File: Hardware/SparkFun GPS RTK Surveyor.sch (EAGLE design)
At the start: 122 parts, among them J13 Internal, J16 microSD, J17 Qwiic Right Angle, J3 USB Female Type C Connector, J4 External, J5 USB Female Type C Connector, Q1 DMC2700UDM, Q10 20V/0.2A/8MHz/1.2Ω/1Vth, Q2 MBT3904DW1T1, Q3 20V/0.2A/8MHz/1.2Ω/1Vth, Q4 20V/0.2A/8MHz/1.2Ω/1Vth, Q7 20V/0.2A/8MHz/1.2Ω/1Vth, Q9 20V/0.2A/8MHz/1.2Ω/1Vth, U1 74HC4052D, U10 MCP73833, U13 9DoF IMU, U14 1.8V/100mA, U2 AP2112K-3.3, U3 U-BLOX_ZED-F9P, U4 ADP160, U5 ESP-WROOM-32NARROW, U6 CH340C, U7 MAX17048

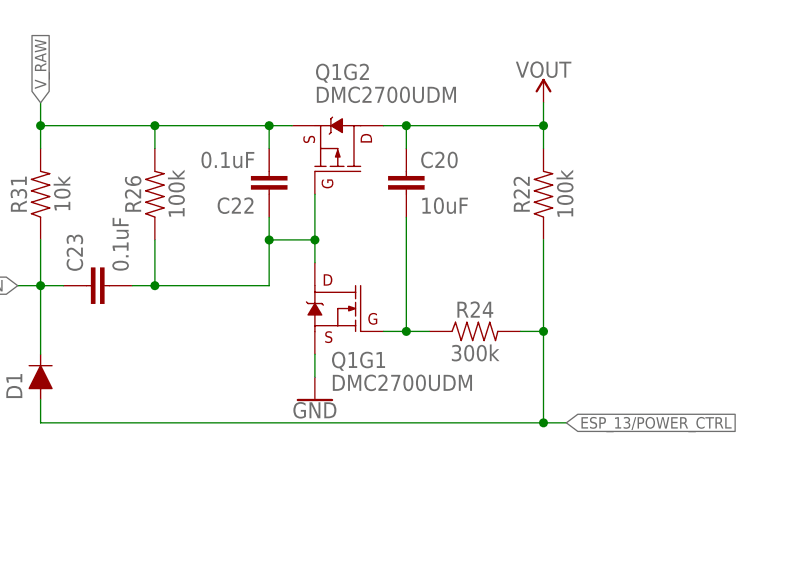
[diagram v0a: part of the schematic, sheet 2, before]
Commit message: Update soft power switch MOSFET
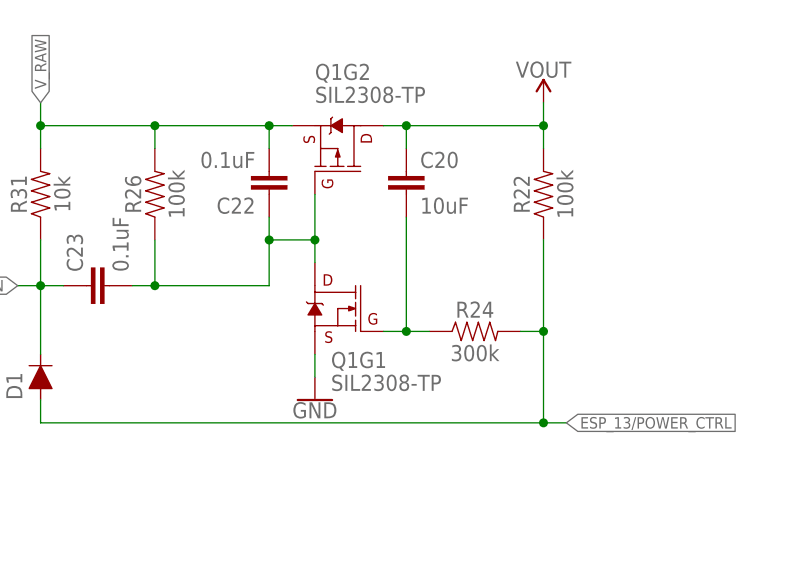
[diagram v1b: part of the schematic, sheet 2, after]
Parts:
- Q1: value DMC2700UDM -> SIL2308-TP; device SparkFun-DiscreteSemi:MOSFET_COMPLIMENTARY_PAIR-DMC2700UDM -> SparkFun-DiscreteSemi:MOSFET_COMPLIMENTARY_PAIR-SIL2308
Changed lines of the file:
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@@
 <part name="R9" library="SparkFun-Resistors" deviceset="33OHM_RA" device="-1206-1/16W-5%" value="33"/>
 <part name="J6" library="SparkFun-Connectors" deviceset="CONN_05" device="NO_SILK"/>
-<part name="Q1" library="SparkFun-DiscreteSemi" deviceset="MOSFET_COMPLIMENTARY_PAIR" device="-DMC2700UDM" value="DMC2700UDM"/>
+<part name="Q1" library="SparkFun-DiscreteSemi" deviceset="MOSFET_COMPLIMENTARY_PAIR" device="-SIL2308" value="SIL2308-TP"/>
 <part name="C20" library="SparkFun-Capacitors" deviceset="10UF" device="-0603-6.3V-20%" value="10uF"/>
 <part name="R22" library="SparkFun-Resistors" deviceset="100KOHM" device="-0603-1/10W-1%" value="100k"/>
